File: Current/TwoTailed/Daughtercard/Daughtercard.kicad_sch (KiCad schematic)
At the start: 6 parts, among them J1 Conn_02x05_Odd_Even, SW1 SW_SPDT, SW2 SW_SPDT, SW3 SW_SPDT, SW4 SW_SPDT, SW5 SW_SPDT

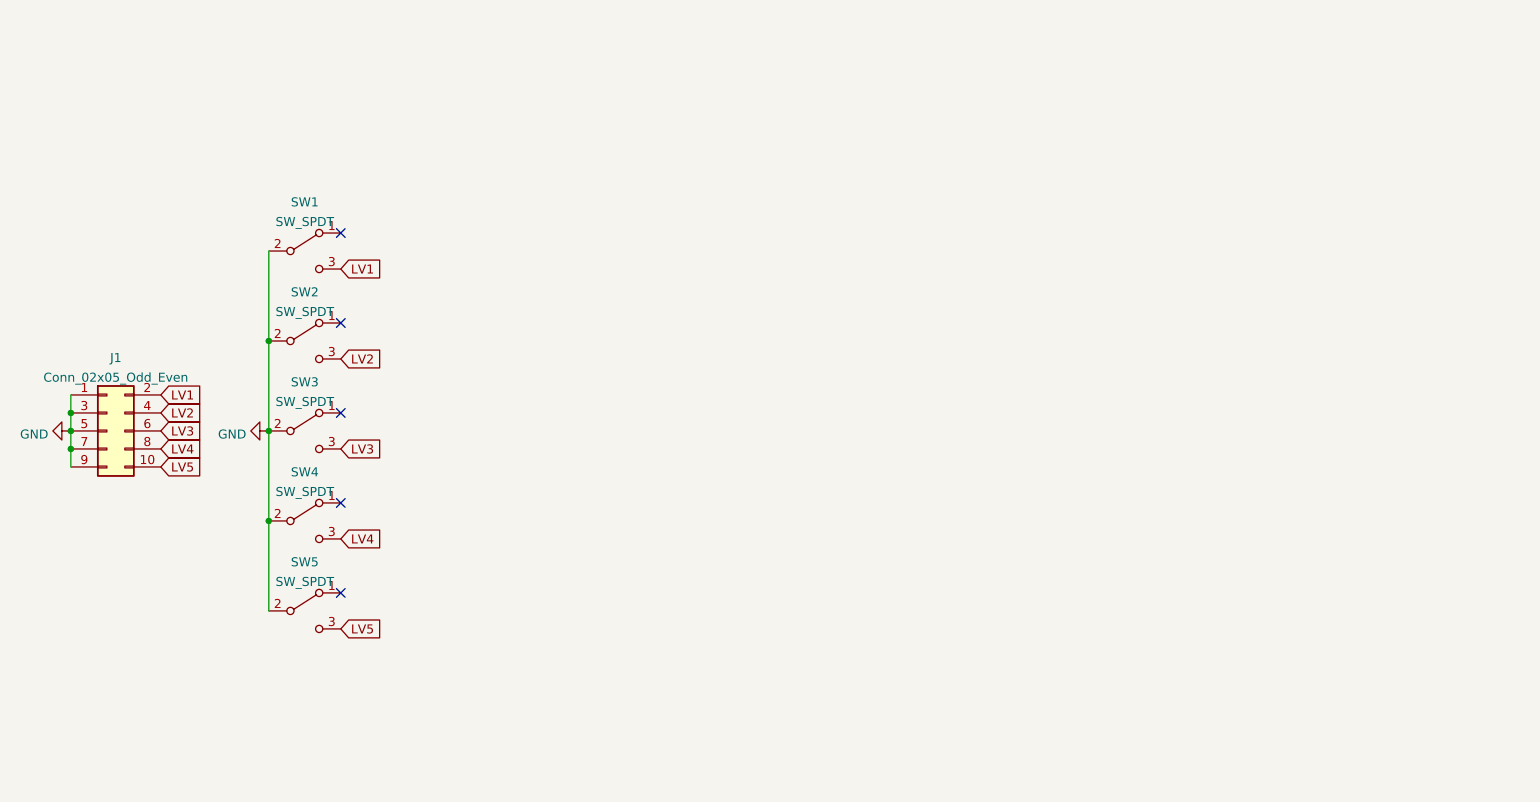
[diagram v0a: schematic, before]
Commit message: So much stuff
Wow it's been a while.
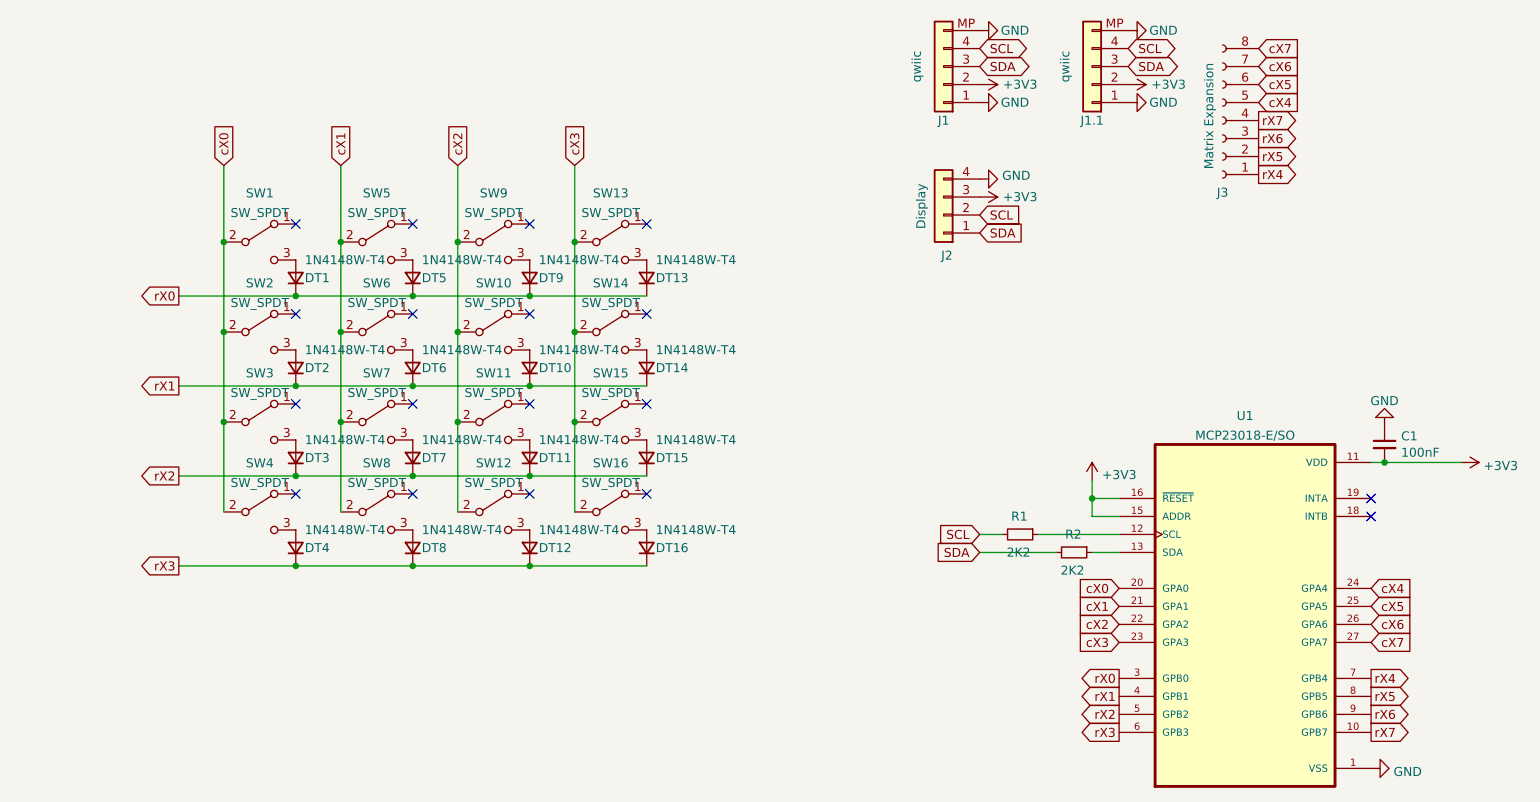
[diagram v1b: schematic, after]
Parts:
- removed J1: Conn_02x05_Odd_Even, Connector_PinHeader_2.54mm:PinHeader_2x05_P2.54mm_Vertical, symbol Connector_Generic:Conn_02x05_Odd_Even
- added C1: 100nF, EDI:Passive_0402_1005Metric, symbol Device:C_Small
- added DT1, DT10, DT11, DT12, DT13, DT14, DT15, DT16, DT2, DT3, DT4, DT5, DT6, DT7, DT8, DT9: 1N4148W-T4, EDI:D_SOD-523, symbol Device:D_Small
- added J1, J1.1: qwiic, Connector_JST:JST_SH_SM04B-SRSS-TB_1x04-1MP_P1.00mm_Horizontal, symbol Connector_Generic:Conn_01x05
- added J2: Display, Connector_PinHeader_2.54mm:PinHeader_1x04_P2.54mm_Vertical, symbol Connector_Generic:Conn_01x04
- added J3: Matrix Expansion, Connector_JST:JST_PH_S8B-PH-K_1x08_P2.00mm_Horizontal, symbol Connector:Conn_01x08_Female
- added R1, R2: 2K2, EDI:Passive_0402_1005Metric, symbol Device:R_Small
- added SW10, SW11, SW12, SW13, SW14, SW15, SW16, SW6, SW7, SW8, SW9: SW_SPDT, EDI:T8013-Z1BQ, symbol Switch:SW_SPDT
- added U1: MCP23018-E/SO, Package_SO:SOIC-28W_7.5x18.7mm_P1.27mm, symbol EDI:MCP23018
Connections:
- net GND: now also C1.1, J1.1 (Pin_1), J1.1.1 (Pin_1), J1.1.MP, J1.MP, J2.4 (Pin_4), U1.1 (VSS); no longer SW1.2 (B), SW2.2 (B), SW3.2 (B), SW4.2 (B), SW5.2 (B)
- net LV1: no longer names the net of SW1.3 (C)
- net LV1: now also DT1.2 (A)
- net LV2: no longer names the net of SW2.3 (C)
- net LV2: now also DT2.2 (A)
- net LV3: no longer names the net of SW3.3 (C)
- net LV3: now also DT3.2 (A)
- net LV4: no longer names the net of SW4.3 (C)
- net LV4: now also DT4.2 (A)
- net LV5: no longer names the net of SW5.3 (C)
- net LV5: now also DT5.2 (A)
- new net: DT6.2 (A), SW6.3 (C)
- new net: DT11.2 (A), SW11.3 (C)
- new net: DT12.2 (A), SW12.3 (C)
- new net: DT8.2 (A), SW8.3 (C)
- new net: DT10.2 (A), SW10.3 (C)
- new net: R1.1, U1.12 (SCL)
- new net: R2.1, U1.13 (SDA)
- new net: DT7.2 (A), SW7.3 (C)
- new net: DT13.2 (A), SW13.3 (C)
- new net: DT14.2 (A), SW14.3 (C)
- new net: DT15.2 (A), SW15.3 (C)
- new net: DT16.2 (A), SW16.3 (C)
- new net: DT9.2 (A), SW9.3 (C)
- new net +3V3: C1.2, J1.1.2 (Pin_2), J1.2 (Pin_2), J2.3 (Pin_3), U1.11 (VDD), U1.15 (ADDR), U1.16 (~{RESET})
- new net SCL: J1.1.4 (Pin_4), J1.4 (Pin_4), J2.2 (Pin_2), R1.2
- new net SDA: J1.1.3 (Pin_3), J1.3 (Pin_3), J2.1 (Pin_1), R2.2
- new net cX0: SW1.2 (B), SW2.2 (B), SW3.2 (B), SW4.2 (B), U1.20 (GPA0)
- new net cX1: SW5.2 (B), SW6.2 (B), SW7.2 (B), SW8.2 (B), U1.21 (GPA1)
- new net cX2: SW10.2 (B), SW11.2 (B), SW12.2 (B), SW9.2 (B), U1.22 (GPA2)
- new net cX3: SW13.2 (B), SW14.2 (B), SW15.2 (B), SW16.2 (B), U1.23 (GPA3)
- new net cX4: J3.5 (Pin_5), U1.24 (GPA4)
- new net cX5: J3.6 (Pin_6), U1.25 (GPA5)
- new net cX6: J3.7 (Pin_7), U1.26 (GPA6)
- new net cX7: J3.8 (Pin_8), U1.27 (GPA7)
- new net rX0: DT1.1 (K), DT13.1 (K), DT5.1 (K), DT9.1 (K), U1.3 (GPB0)
- new net rX1: DT10.1 (K), DT14.1 (K), DT2.1 (K), DT6.1 (K), U1.4 (GPB1)
- new net rX2: DT11.1 (K), DT15.1 (K), DT3.1 (K), DT7.1 (K), U1.5 (GPB2)
- new net rX3: DT12.1 (K), DT16.1 (K), DT4.1 (K), DT8.1 (K), U1.6 (GPB3)
- new net rX4: J3.1 (Pin_1), U1.7 (GPB4)
- new net rX5: J3.2 (Pin_2), U1.8 (GPB5)
- new net rX6: J3.3 (Pin_3), U1.9 (GPB6)
- new net rX7: J3.4 (Pin_4), U1.10 (GPB7)
- no-connect marks 5 -> 18
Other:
- moved on the sheet: SW1, SW2, SW3, SW4
